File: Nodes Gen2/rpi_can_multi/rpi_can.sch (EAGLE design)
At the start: 37 parts, among them IC1 DS1820TO92, IC2 MCP2551, IC3 MAX481CSA, IC4 MCP2551, K4 615016240521

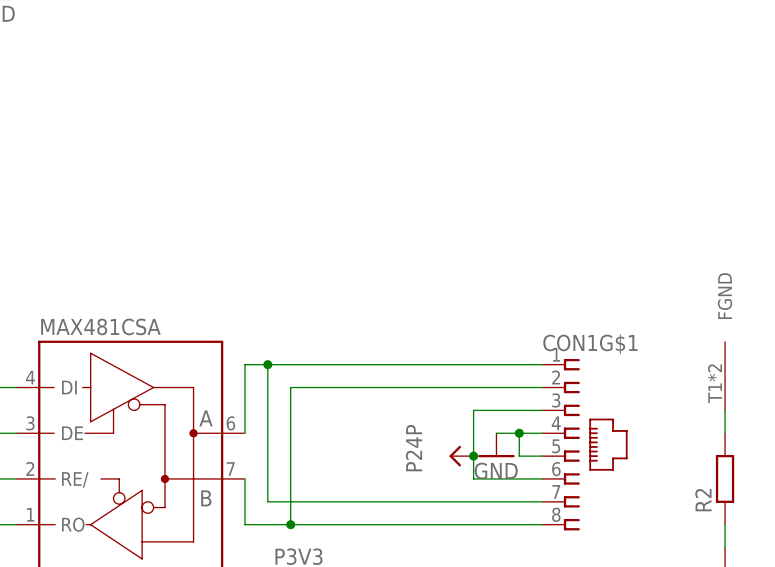
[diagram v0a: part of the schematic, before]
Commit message: so much...
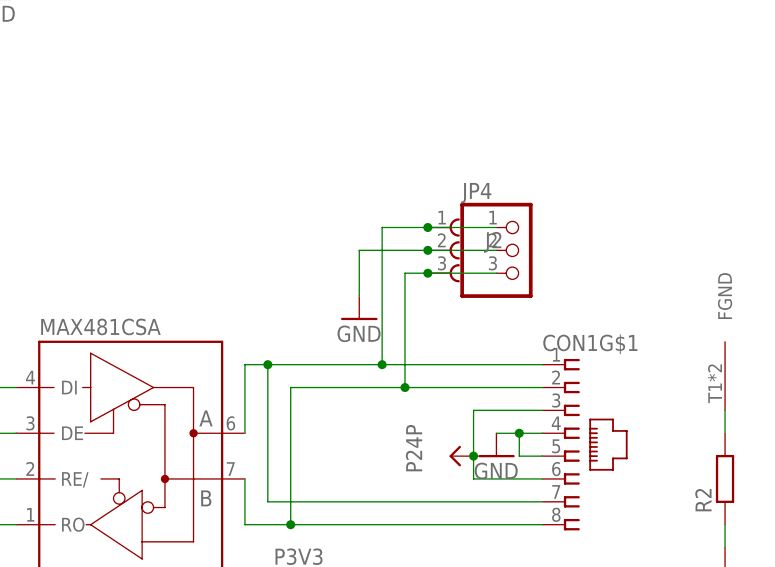
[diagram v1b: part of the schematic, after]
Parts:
- added J2: (no value), Wuerth_TERMINAL_BLOCKS_rev16a:691322310003
- added JP4: (no value), pinhead:PINHD-1X3
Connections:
- net GND: now also J2.2, JP4.2
- net RS485_A: now also J2.1, JP4.1
- net RS485_B: now also J2.3, JP4.3
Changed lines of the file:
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@@
 <part name="SUPPLY20" library="schlager_supply" deviceset="P24P" device=""/>
 <part name="GND22" library="supply1" deviceset="GND" device=""/>
+<part name="J2" library="Wuerth_TERMINAL_BLOCKS_rev16a" deviceset="691322310003" device=""/>
+<part name="GND23" library="supply1" deviceset="GND" device=""/>
+<part name="JP4" library="pinhead" deviceset="PINHD-1X3" device=""/>
 </parts>
 <sheets>
@@
 <instance part="SUPPLY20" gate="G$1" x="276.86" y="215.9" rot="R90"/>
 <instance part="GND22" gate="1" x="279.4" y="208.28"/>
+<instance part="J2" gate="G$1" x="332.74" y="180.34"/>
+<instance part="GND23" gate="1" x="320.04" y="172.72"/>
+<instance part="JP4" gate="A" x="337.82" y="180.34"/>
 </instances>
 <busses>
@@
 <wire x1="281.94" y1="213.36" x2="279.4" y2="210.82" width="0.1524" layer="91"/>
 </segment>
+<segment>
+<pinref part="J2" gate="G$1" pin="2"/>
+<pinref part="GND23" gate="1" pin="GND"/>
+<wire x1="327.66" y1="180.34" x2="320.04" y2="180.34" width="0.1524" layer="91"/>
+<wire x1="320.04" y1="180.34" x2="320.04" y2="175.26" width="0.1524" layer="91"/>
+<pinref part="JP4" gate="A" pin="2"/>
+<wire x1="327.66" y1="180.34" x2="335.28" y2="180.34" width="0.1524" layer="91"/>
+<junction x="327.66" y="180.34"/>
+</segment>
 </net>
 <net name="P5V" class="0">
@@
 <wire x1="309.88" y1="152.4" x2="309.88" y2="167.64" width="0.1524" layer="91"/>
 <pinref part="CON1" gate="G$1" pin="1"/>
-<wire x1="309.88" y1="167.64" x2="340.36" y2="167.64" width="0.1524" layer="91"/>
+<wire x1="309.88" y1="167.64" x2="322.58" y2="167.64" width="0.1524" layer="91"/>
 <junction x="309.88" y="167.64"/>
+<pinref part="J2" gate="G$1" pin="1"/>
+<wire x1="322.58" y1="167.64" x2="340.36" y2="167.64" width="0.1524" layer="91"/>
+<wire x1="327.66" y1="182.88" x2="322.58" y2="182.88" width="0.1524" layer="91"/>
+<wire x1="322.58" y1="182.88" x2="322.58" y2="167.64" width="0.1524" layer="91"/>
+<junction x="322.58" y="167.64"/>
+<pinref part="JP4" gate="A" pin="1"/>
+<wire x1="335.28" y1="182.88" x2="327.66" y2="182.88" width="0.1524" layer="91"/>
+<junction x="327.66" y="182.88"/>
 </segment>
 </net>
@@
 <segment>
 <pinref part="CON1" gate="G$1" pin="2"/>
-<wire x1="340.36" y1="165.1" x2="312.42" y2="165.1" width="0.1524" layer="91"/>
+<wire x1="340.36" y1="165.1" x2="325.12" y2="165.1" width="0.1524" layer="91"/>
 <pinref part="CON1" gate="G$1" pin="8"/>
+<wire x1="325.12" y1="165.1" x2="312.42" y2="165.1" width="0.1524" layer="91"/>
 <wire x1="307.34" y1="149.86" x2="312.42" y2="149.86" width="0.1524" layer="91"/>
 <pinref part="IC3" gate="G$1" pin="B"/>
@@
 <wire x1="312.42" y1="165.1" x2="312.42" y2="149.86" width="0.1524" layer="91"/>
 <junction x="312.42" y="149.86"/>
-</segment>
-</net>
+<pinref part="J2" gate="G$1" pin="3"/>
+<wire x1="327.66" y1="177.8" x2="325.12" y2="177.8" width="0.1524" layer="91"/>
+<wire x1="325.12" y1="177.8" x2="325.12" y2="165.1" width="0.1524" layer="91"/>
+<junction x="325.12" y="165.1"/>
+<pinref part="JP4" gate="A" pin="3"/>
+<wire x1="335.28" y1="177.8" x2="327.66" y2="177.8" width="0.1524" layer="91"/>
+<junction x="327.66" y="177.8"/>
+</segment>
+</net>
